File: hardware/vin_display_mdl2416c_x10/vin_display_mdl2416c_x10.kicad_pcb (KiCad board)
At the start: 2 copper layers, 221 x 83.8 mm, 61 parts, among them J1 DEBUG, J2 USB_B_Micro, J3 DEBUG_UART, J4 IF_UART, J5 AUX_CONNECTOR, Q1 BSS138, SW1 SW_RESET, SW2 BOOTSEL, SW3 KNOB, U1 W25Q16JVSNIQ, U10 MDL2416C, U11 MDL2416C, U12 MDL2416C, U13 MDL2416C, U14 MDL2416C, U2 MIC23050-SYML, U3 RP2040, U4 HEF4028BT, U5 MDL2416C, U6 MDL2416C, U7 MDL2416C, U8 MDL2416C, U9 MDL2416C, X1 12MHz

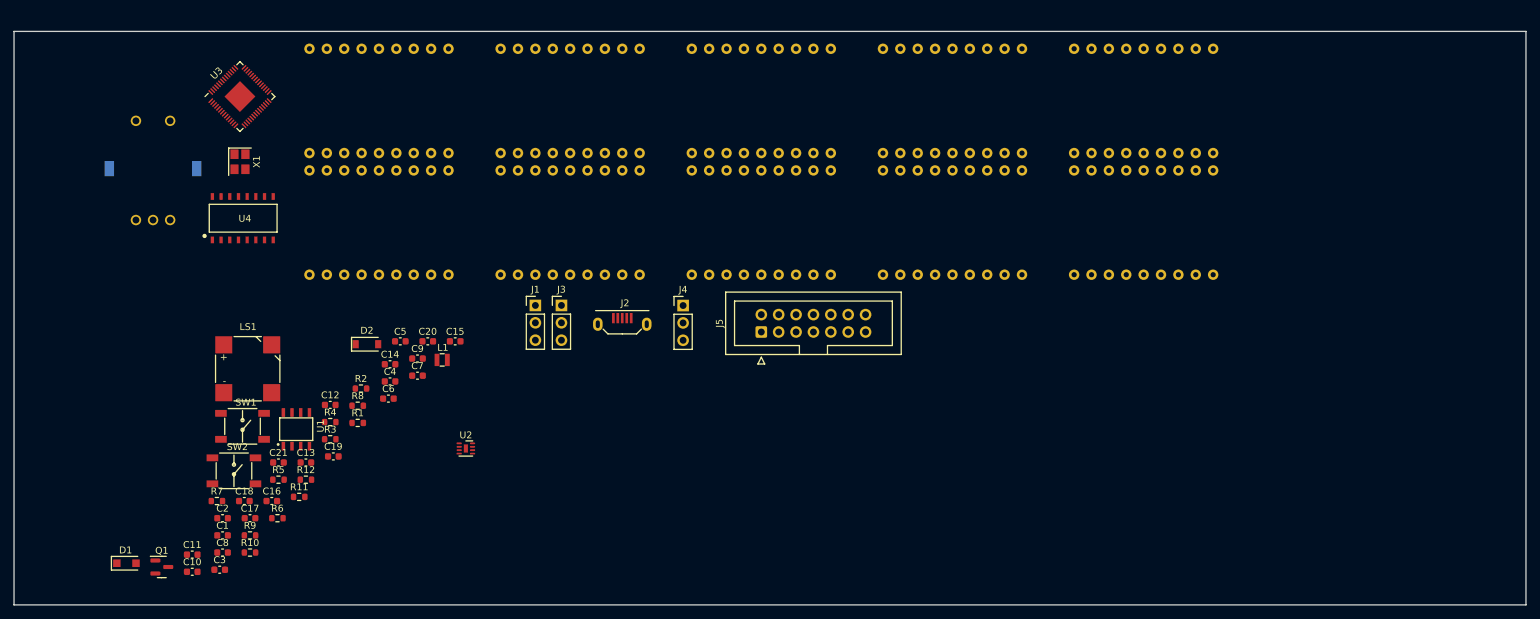
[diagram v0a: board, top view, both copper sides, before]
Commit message: work on pcb layout
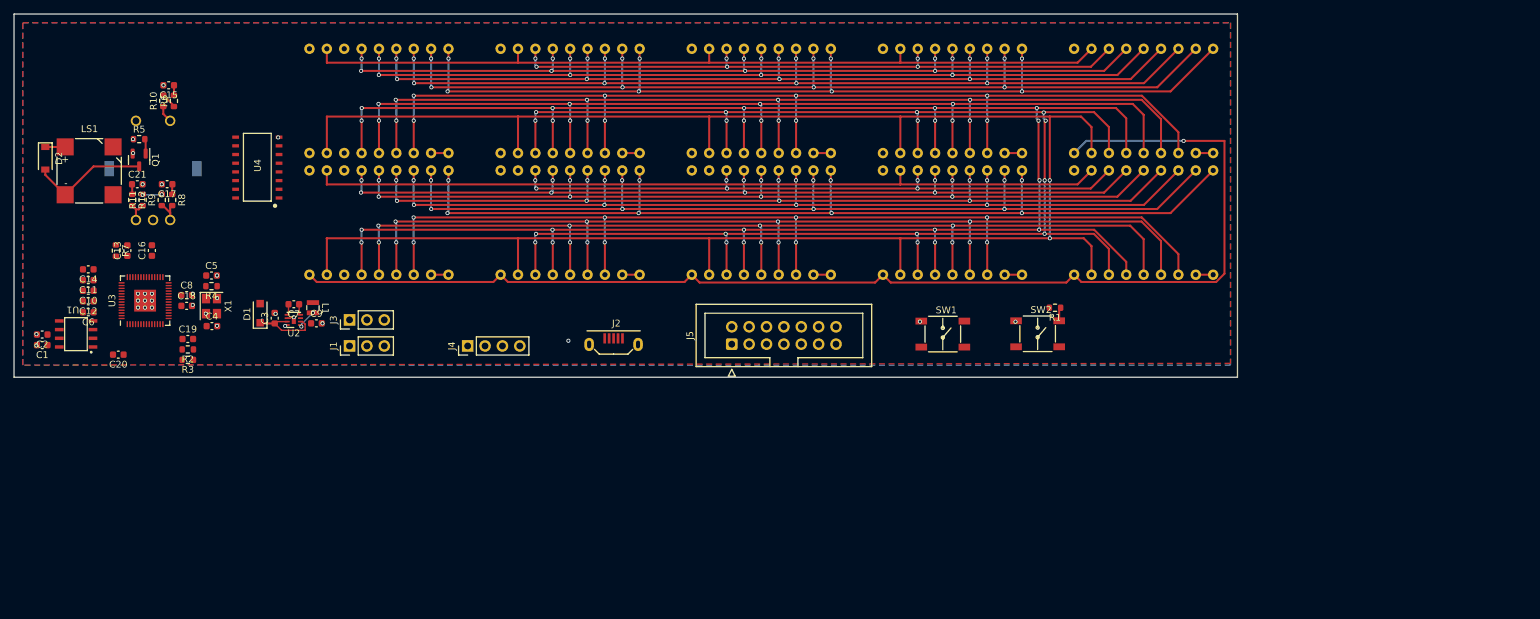
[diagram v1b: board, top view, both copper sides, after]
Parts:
- J4: value IF_UART -> Conn_01x04; footprint Connector_PinHeader_2.54mm:PinHeader_1x03_P2.54mm_Vertical -> Connector_PinHeader_2.54mm:PinHeader_1x04_P2.54mm_Vertical
- moved SW2 119.2 mm to (175.0, 95.0)
- moved R1 103.3 mm to (177.5, 91.2), turned to 180 degrees
- moved SW1 103.2 mm to (161.1, 95.0)
- moved R10 67.2 mm to (47.2, 61.0), turned to 90 degrees
- moved R6 62.8 mm to (48.8, 61.0), turned to 90 degrees
- moved Q1 59.6 mm to (43.7, 69.6), turned to -90 degrees
- moved C15 56.2 mm to (48.0, 58.7), turned to 180 degrees
- moved D2 54.3 mm to (30.0, 69.3), turned to -90 degrees
- moved R5 53.8 mm to (43.7, 66.5)
- moved R9 50.7 mm to (47.0, 75.4), turned to 90 degrees
- moved C17 50.3 mm to (47.8, 73.1), turned to 180 degrees
- moved R11 49.1 mm to (44.2, 75.4), turned to 90 degrees
- moved R12 48.1 mm to (42.7, 75.4), turned to -90 degrees
- moved C14 46.2 mm to (36.3, 85.6), turned to 180 degrees
- moved C6 45.6 mm to (36.3, 91.9), turned to 180 degrees
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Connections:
- net Net-(R2-Pad2) renamed USB_D+
- net Net-(R3-Pad2) renamed USB_D-
- C1 pad 1: Net-(C1-Pad1) -> 3V3
- C2 pad 1: Net-(C1-Pad1) -> 3V3
- J4 pad 1: UART1_TX -> VSYS
- J4 pad 2: GND -> UART1_TX
- J4 pad 3: UART1_RX -> GND
- U1 pad 8: Net-(C1-Pad1) -> 3V3
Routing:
- net DISP_WR: track 0.00 -> 304.0 mm, vias 0 -> 20
- net DISP_CLR: track 0.00 -> 301.1 mm, vias 0 -> 16
- net DISP_CUE: track 0.00 -> 298.5 mm, vias 0 -> 16
- net DISP_CU: track 0.00 -> 293.7 mm, vias 0 -> 16
- net DISP_A0: track 0.00 -> 293.1 mm, vias 0 -> 2
- net DISP_BL: track 0.00 -> 279.2 mm, vias 0 -> 16
- net DISP_D4: track 0.00 -> 273.3 mm, vias 0 -> 16
- net DISP_D5: track 0.00 -> 268.0 mm, vias 0 -> 16
- net DISP_D6: track 0.00 -> 262.8 mm, vias 0 -> 16
- net DISP_D3: track 0.00 -> 257.5 mm, vias 0 -> 16
- net DISP_D2: track 0.00 -> 252.6 mm, vias 0 -> 16
- net DISP_D0: track 0.00 -> 237.4 mm
- net DISP_A1: track 0.00 -> 231.2 mm, vias 0 -> 16
- net VSYS: track 0.00 -> 194.1 mm, vias 0 -> 1
- net DISP_D1: track 0.00 -> 185.6 mm, vias 0 -> 12
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- added copper zone on F.Cu, net 3V3
- added copper zone on B.Cu, net GND
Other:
- board size 221 x 83.8 mm -> 178.8 x 53.1 mm
